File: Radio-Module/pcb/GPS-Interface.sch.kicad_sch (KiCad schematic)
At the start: 3 parts, among them U1 MAX-8C

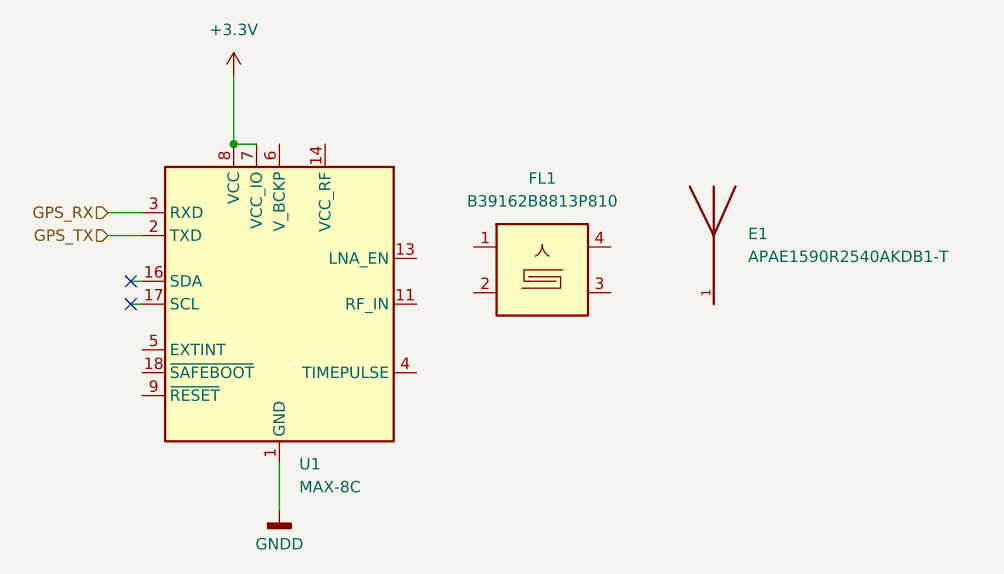
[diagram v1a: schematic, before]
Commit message: Finished radio module
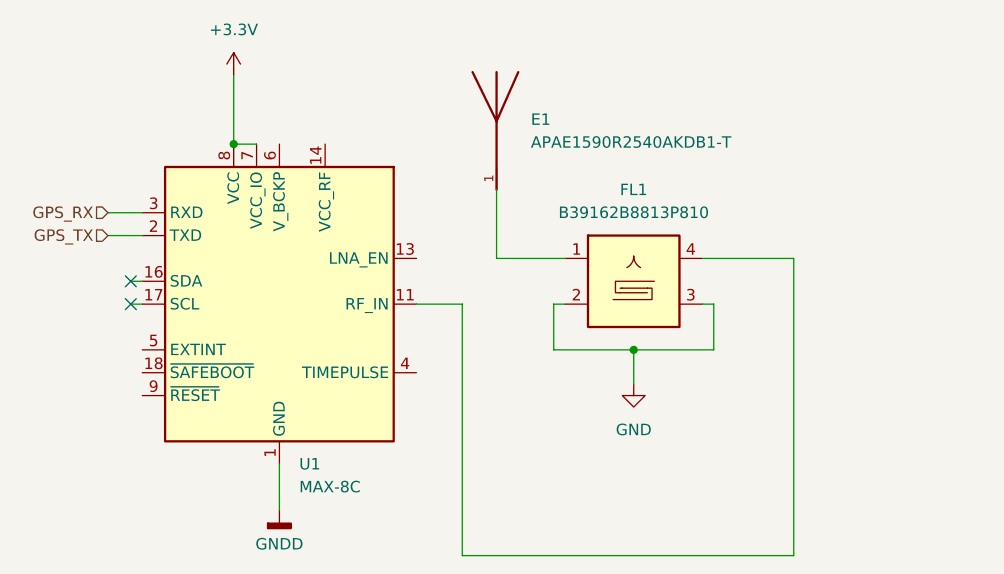
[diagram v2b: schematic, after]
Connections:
- net at FL1.1: now also E1.1
- net GND: now reaches FL1.2, FL1.5
- net GND: now also FL1.3
- net at FL1.4: now also U1.11 (RF_IN)
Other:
- moved on the sheet: E1, FL1
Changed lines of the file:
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@@
 	(paper "A4")
+	(junction
+		(at 171.45 102.87)
+		(diameter 0)
+		(color 0 0 0 0)
+	)
 	(junction
 		(at 127 80.01)
@@
 	(wire
 		(pts
+			(xy 162.56 97.79) (xy 162.56 102.87)
+		)
+		(stroke
+			(width 0)
+			(type default)
+		)
+	)
+	(wire
+		(pts
 			(xy 115.57 95.25) (xy 116.84 95.25)
 		)
@@
 	(wire
 		(pts
+			(xy 189.23 125.73) (xy 189.23 92.71)
+		)
+		(stroke
+			(width 0)
+			(type default)
+		)
+	)
+	(wire
+		(pts
+			(xy 152.4 97.79) (xy 152.4 125.73)
+		)
+		(stroke
+			(width 0)
+			(type default)
+		)
+	)
+	(wire
+		(pts
 			(xy 113.03 87.63) (xy 116.84 87.63)
 		)
@@
 	(wire
 		(pts
+			(xy 180.34 97.79) (xy 179.07 97.79)
+		)
+		(stroke
+			(width 0)
+			(type default)
+		)
+	)
+	(wire
+		(pts
+			(xy 189.23 92.71) (xy 179.07 92.71)
+		)
+		(stroke
+			(width 0)
+			(type default)
+		)
+	)
+	(wire
+		(pts
 			(xy 127 72.39) (xy 127 80.01)
 		)
@@
 	(wire
 		(pts
+			(xy 171.45 102.87) (xy 180.34 102.87)
+		)
+		(stroke
+			(width 0)
+			(type default)
+		)
+	)
+	(wire
+		(pts
+			(xy 180.34 102.87) (xy 180.34 97.79)
+		)
+		(stroke
+			(width 0)
+			(type default)
+		)
+	)
+	(wire
+		(pts
+			(xy 163.83 92.71) (xy 156.21 92.71)
+		)
+		(stroke
+			(width 0)
+			(type default)
+		)
+	)
+	(wire
+		(pts
+			(xy 163.83 97.79) (xy 162.56 97.79)
+		)
+		(stroke
+			(width 0)
+			(type default)
+		)
+	)
+	(wire
+		(pts
+			(xy 152.4 125.73) (xy 189.23 125.73)
+		)
+		(stroke
+			(width 0)
+			(type default)
+		)
+	)
+	(wire
+		(pts
+			(xy 156.21 85.09) (xy 156.21 92.71)
+		)
+		(stroke
+			(width 0)
+			(type default)
+		)
+	)
+	(wire
+		(pts
 			(xy 115.57 97.79) (xy 116.84 97.79)
+		)
+		(stroke
+			(width 0)
+			(type default)
+		)
+	)
+	(wire
+		(pts
+			(xy 171.45 102.87) (xy 171.45 106.68)
+		)
+		(stroke
+			(width 0)
+			(type default)
+		)
+	)
+	(wire
+		(pts
+			(xy 147.32 97.79) (xy 152.4 97.79)
+		)
+		(stroke
+			(width 0)
+			(type default)
+		)
+	)
+	(wire
+		(pts
+			(xy 162.56 102.87) (xy 171.45 102.87)
 		)
 		(stroke
@@
 	(symbol
 		(lib_id "Filter:B39162B8813P810")
-		(at 161.29 93.98 0)
+		(at 171.45 95.25 0)
 		(unit 1)
 		(exclude_from_sim no)
@@
 		(fields_autoplaced yes)
 		(property "Reference" "FL1"
-			(at 161.29 83.82 0)
+			(at 171.45 85.09 0)
 			(effects
 				(font
@@
 		)
 		(property "Value" "B39162B8813P810"
-			(at 161.29 86.36 0)
+			(at 171.45 87.63 0)
 			(effects
 				(font
@@
 		)
 		(property "Footprint" "Filter:Filter_1109-5_1.1x0.9mm"
-			(at 161.29 93.98 0)
+			(at 171.45 95.25 0)
 			(effects
 				(font
@@
 		)
 		(property "Datasheet" "https://product.tdk.com/search-template/en/documents/data_sheet/40/ds/mc/B9482.pdf"
-			(at 159.512 93.218 0)
+			(at 169.672 94.488 0)
 			(effects
 				(font
@@
 		)
 		(property "Description" "1582.47MHz SAW filter, SMD 1109"
-			(at 161.29 93.98 0)
+			(at 171.45 95.25 0)
 			(effects
 				(font
@@
 	)
 	(symbol
+		(lib_id "power:GND")
+		(at 171.45 106.68 0)
+		(unit 1)
+		(exclude_from_sim no)
+		(in_bom yes)
+		(on_board yes)
+		(dnp no)
+		(fields_autoplaced yes)
+		(property "Reference" "#PWR031"
+			(at 171.45 113.03 0)
+			(effects
+				(font
+					(size 1.27 1.27)
+				)
+				(hide yes)
+			)
+		)
+		(property "Value" "GND"
+			(at 171.45 111.76 0)
+			(effects
+				(font
+					(size 1.27 1.27)
+				)
+			)
+		)
+		(property "Footprint" ""
+			(at 171.45 106.68 0)
+			(effects
+				(font
+					(size 1.27 1.27)
+				)
+				(hide yes)
+			)
+		)
+		(property "Datasheet" ""
+			(at 171.45 106.68 0)
+			(effects
+				(font
+					(size 1.27 1.27)
+				)
+				(hide yes)
+			)
+		)
+		(property "Description" "Power symbol creates a global label with name \"GND\" , ground"
+			(at 171.45 106.68 0)
+			(effects
+				(font
+					(size 1.27 1.27)
+				)
+				(hide yes)
+			)
+		)
+		(pin "1"
+		)
+		(instances
+			(project ""
+				(path "/acc63f22-7eb8-450a-9af4-da5f4b8157d9/f4383c06-cfae-4b6b-8591-014188dc9624"
+					(reference "#PWR031")
+					(unit 1)
+				)
+			)
+		)
+	)
+	(symbol
 		(lib_id "APAE1590R2540AKDB1-T:APAE1590R2540AKDB1-T")
-		(at 180.34 92.71 0)
+		(at 156.21 80.01 0)
 		(unit 1)
 		(exclude_from_sim no)
@@
 		(fields_autoplaced yes)
 		(property "Reference" "E1"
-			(at 184.15 89.9794 0)
+			(at 160.02 77.2794 0)
 			(effects
 				(font
@@
 		)
 		(property "Value" "APAE1590R2540AKDB1-T"
-			(at 184.15 92.5194 0)
+			(at 160.02 79.8194 0)
 			(effects
 				(font
@@
 		)
 		(property "Footprint" "APAE1590R2540AKDB1_T:XDCR_APAE1590R2540AKDB1-T"
-			(at 180.34 92.71 0)
+			(at 156.21 80.01 0)
 			(effects
 				(font
@@
 		)
 		(property "Datasheet" ""
-			(at 180.34 92.71 0)
+			(at 156.21 80.01 0)
 			(effects
 				(font
@@
 		)
 		(property "Description" ""
-			(at 180.34 92.71 0)
+			(at 156.21 80.01 0)
 			(effects
 				(font
@@
 		)
 		(property "PARTREV" "-"
-			(at 180.34 92.71 0)
+			(at 156.21 80.01 0)
 			(effects
 				(font
@@
 		)
 		(property "SNAPEDA_PN" "APAE1590R2540AKDB1-T"
-			(at 180.34 92.71 0)
+			(at 156.21 80.01 0)
 			(effects
 				(font
@@
 		)
 		(property "STANDARD" "IPC-7351B"
-			(at 180.34 92.71 0)
+			(at 156.21 80.01 0)
 			(effects
 				(font
@@
 		)
 		(property "MAXIMUM_PACKAGE_HEIGHT" "4.7mm"
-			(at 180.34 92.71 0)
+			(at 156.21 80.01 0)
 			(effects
 				(font
@@
 		)
 		(property "MANUFACTURER" "Abracon"
-			(at 180.34 92.71 0)
-			(effects
-				(font
+			(at 156.21 80.01 0)
+			(effects
+				(font
